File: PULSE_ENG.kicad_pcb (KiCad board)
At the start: 4 copper layers, 143 parts, among them IC1 TPS7B8733QDDARQ1, IC2 TPS7B8750QDDARQ1, IC28 INA226AIDGSR, IC29 TPS25940ARVCR, IC30 TPS25940ARVCR, IC31 INA226AIDGSR, J10 Screw_Terminal_01x01, J11 Screw_Terminal_01x04, J8 Screw_Terminal_01x04, J9 Screw_Terminal_01x06, U1 ATSAMD21J17D-M, U2 LT6108IMS8-1-TRPBF, U3 LM139ADRG4, U4 EPC2152, U5 LT6108IMS8-1-TRPBF

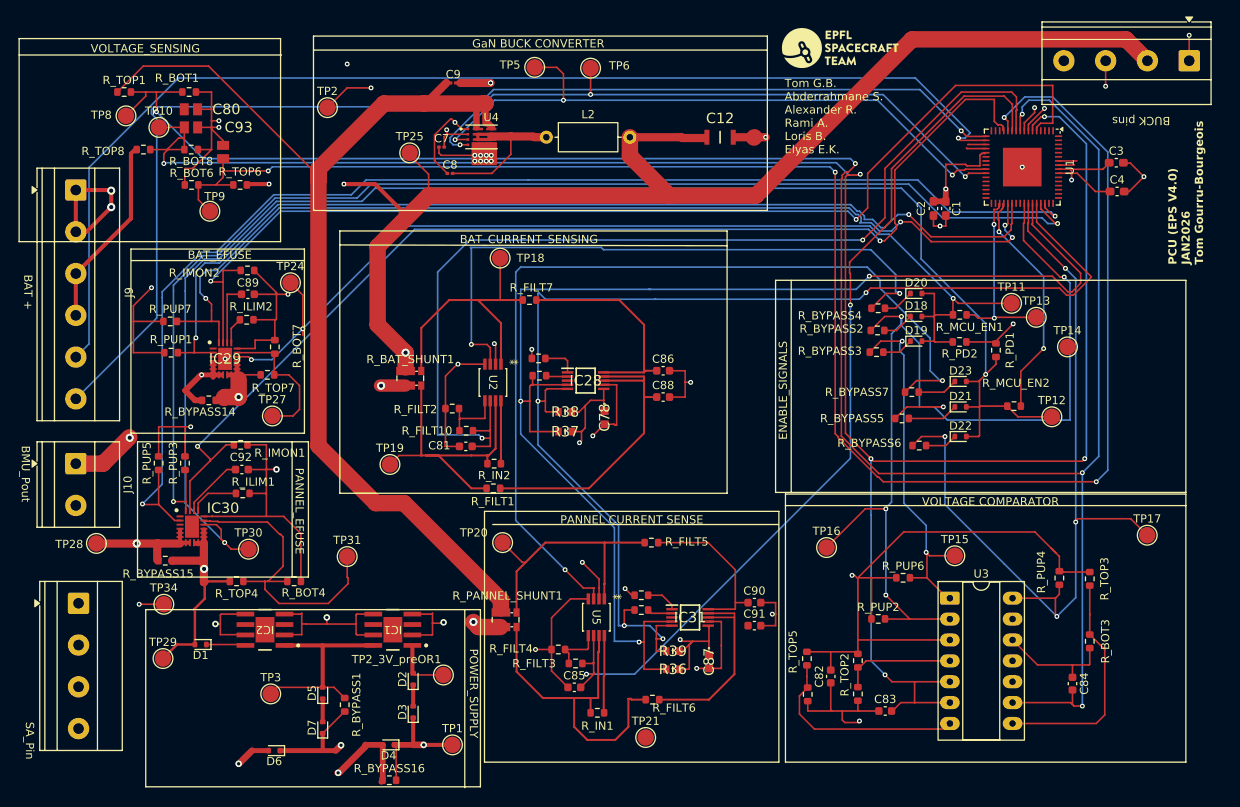
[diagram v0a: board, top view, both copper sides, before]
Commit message: Modofications asked and BOM
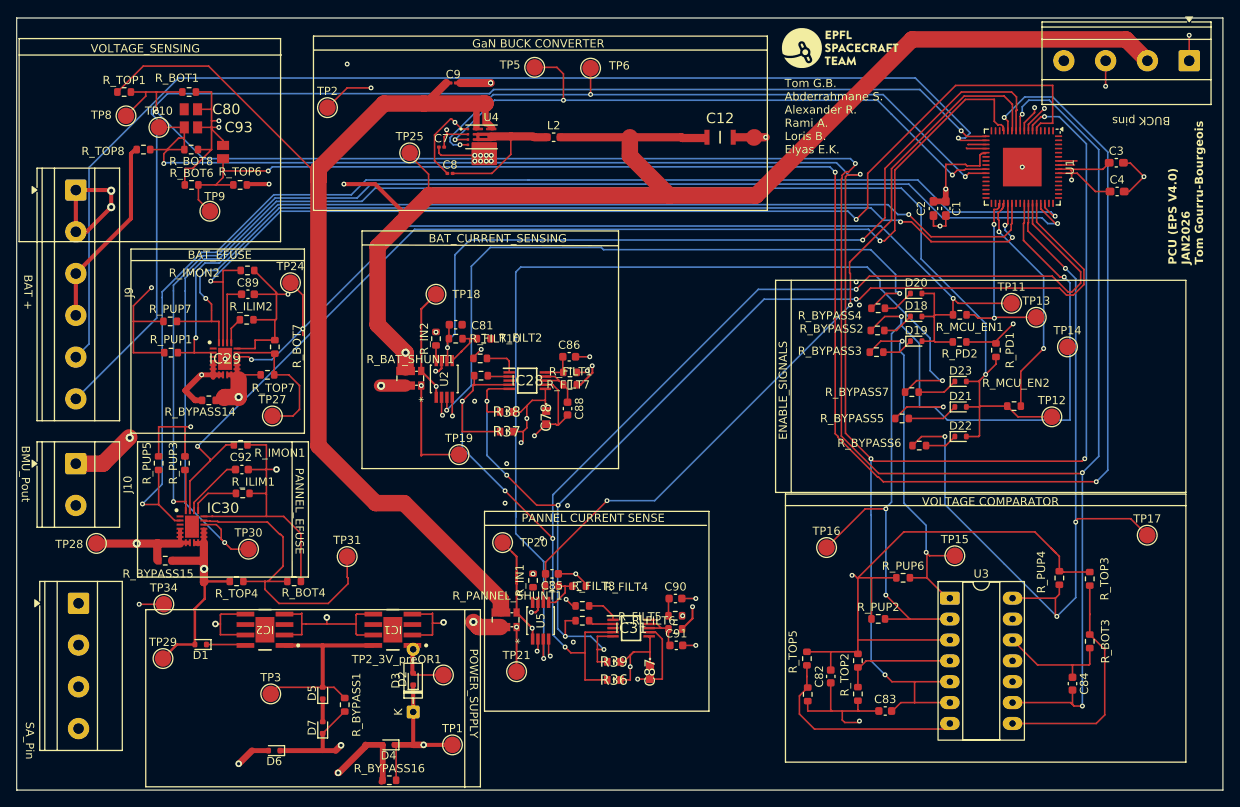
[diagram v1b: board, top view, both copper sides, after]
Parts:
- D3: value 1N4148WT -> 1N5711; footprint Diode_SMD:D_SOD-523 -> Diode_THT:D_DO-35_SOD27_P7.62mm_Horizontal
- L2: footprint Inductor_THT:L_Axial_L7.0mm_D3.3mm_P10.16mm_Horizontal_Fastron_MICC -> Inductor_SMD:L_0603_1608Metric
- moved R_IN1 17.9 mm to (92.2, 124.6), turned to 90 degrees
- moved TP21 17.6 mm to (90.2, 135.7)
- moved R_IN2 16.8 mm to (80.4, 95.2), turned to 90 degrees
- moved R_FILT1 15.7 mm to (96.7, 100.8), turned to 180 degrees
- moved C81 14.9 mm to (82.8, 93.5), turned to 180 degrees
- moved C85 14.1 mm to (94.5, 123.8), turned to 180 degrees
- moved C88 11.7 mm to (96.4, 103.7), turned to -90 degrees
- moved C86 11.6 mm to (96.6, 97.4)
- moved R_FILT10 11.3 mm to (82.8, 95.2), turned to 180 degrees
- moved R_FILT7 10.1 mm to (96.7, 99.3), turned to 180 degrees
- moved R_FILT3 9.83 mm to (94.5, 125.3), turned to 180 degrees
- moved C91 9.80 mm to (109.6, 132.5)
- moved C90 9.61 mm to (109.5, 126.8)
- moved R_FILT5 9.36 mm to (109.5, 128.9), turned to 180 degrees
- moved R_FILT2 9.32 mm to (86.2, 95.2), turned to 180 degrees
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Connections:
- C1 pad 1: VDDIN -> VDDIO
- C2 pad 1: VDDIN -> VDDIO
- C3 pad 1: VDDIN -> VDDIO
- C4 pad 1: VDDIN -> VDDIO
- C82 pad 1: VDDIN -> VDDIO
- C87 pad 1: VDDIN -> VDDIO
- D3 pad 1: VDDIN -> /5V
- D3 pad 2: Net-(D2-K) -> Net-(D3-A)
- D4 pad 1: VDDIN -> VDDIO
- D5 pad 1: Net-(D5-K) -> Net-(D3-A)
- IC31 pad 6: VDDIN -> VDDIO
- R36 pad 2: VDDIN -> VDDIO
- R39 pad 2: VDDIN -> VDDIO
- R_BYPASS16 pad 2: VDDIN -> VDDIO
- R_PUP2 pad 1: VDDIN -> VDDIO
- R_PUP3 pad 2: VDDIN -> VDDIO
- R_PUP4 pad 2: VDDIN -> VDDIO
- R_PUP5 pad 2: VDDIN -> VDDIO
- R_PUP6 pad 1: VDDIN -> VDDIO
- R_TOP2 pad 2: VDDIN -> VDDIO
- R_TOP3 pad 2: VDDIN -> VDDIO
- R_TOP5 pad 2: VDDIN -> VDDIO
- TP1 pad 1: VDDIN -> VDDIO
- U1 pad 21: VDDIN -> VDDIO
- U1 pad 56: VDDIN -> VDDIO
- U1 pad 8: VDDIN -> VDDIO
- U2 pad 2: VDDIN -> VDDIO
- U3 pad 3: VDDIN -> VDDIO
- U5 pad 2: VDDIN -> VDDIO
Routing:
- net Net-(IC28-IN-): track 38.6 -> 6.61 mm
- net GND: track 276.6 -> 244.7 mm, vias 34 -> 44
- net /I_BAT_ANA: track 123.7 -> 100.6 mm
- net Net-(IC28-IN+): track 26.7 -> 4.10 mm
- net Net-(IC31-IN+): track 20.4 -> 2.13 mm
- net Net-(IC31-IN-): track 24.2 -> 6.15 mm
- net /I_PANNEL_ANA: track 111.6 -> 95.8 mm
- net Net-(U5-SENSEHI): track 9.45 -> 0.00 mm
- net /3.3V: track 569.7 -> 560.3 mm, vias 11 -> 12
- net /Vout_BUCK: track 205.9 -> 214.4 mm
- net /PCU_Control/PANNEL_OVC: track 110.7 -> 117.9 mm
- net /BAT_SHUNT_IN: track 38.0 -> 44.9 mm, vias 0 -> 4
- net Net-(U2-SENSEHI): track 7.64 -> 1.86 mm
- net /PANNEL_SHUNT_IN: track 43.3 -> 37.8 mm, vias 0 -> 4
- net SCL2: track 149.8 -> 144.6 mm, vias 4 -> 6
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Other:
- board outline added: 146.7 x 93.9 mm
